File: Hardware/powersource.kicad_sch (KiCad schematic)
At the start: 39 parts, among them J10 USB_C_Receptacle_USB2.0_16P, J14 Conn_01x01_Socket, J15 Conn_01x01_Socket, J6 Conn_01x01_Socket, J9 Conn_01x01_Socket, Q2 DMP3015LSS-13, SW1 SW_Push_DPDT, U4 TPS61022, U8 CN3158

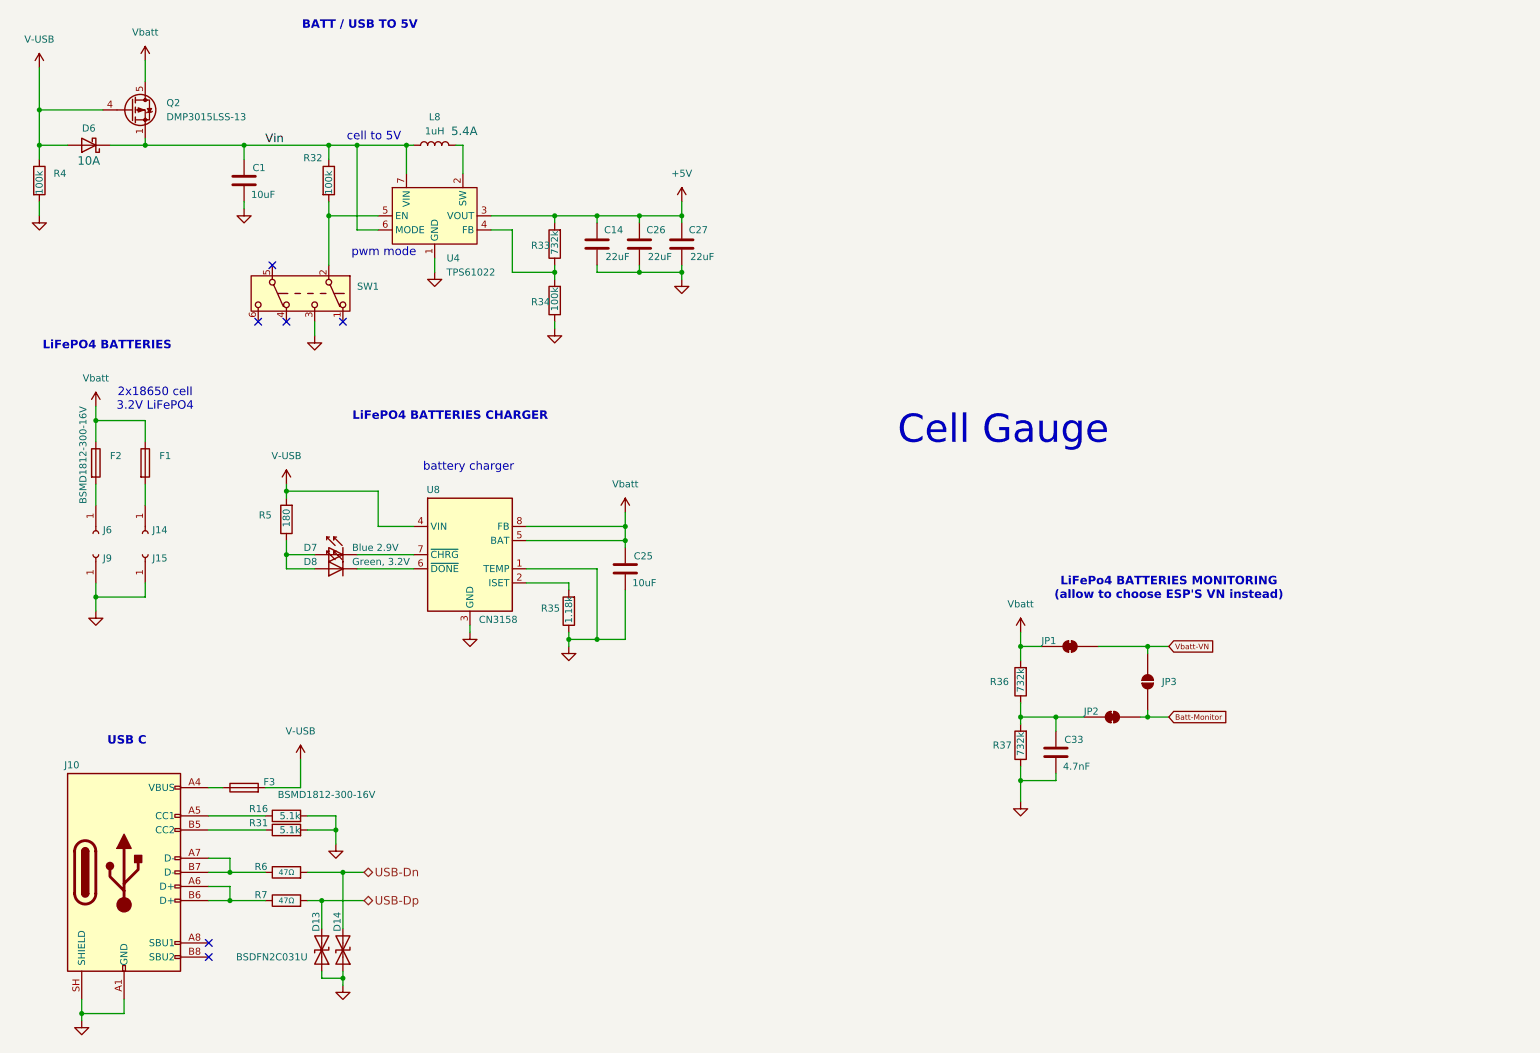
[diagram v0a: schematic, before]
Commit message: Schematic Done
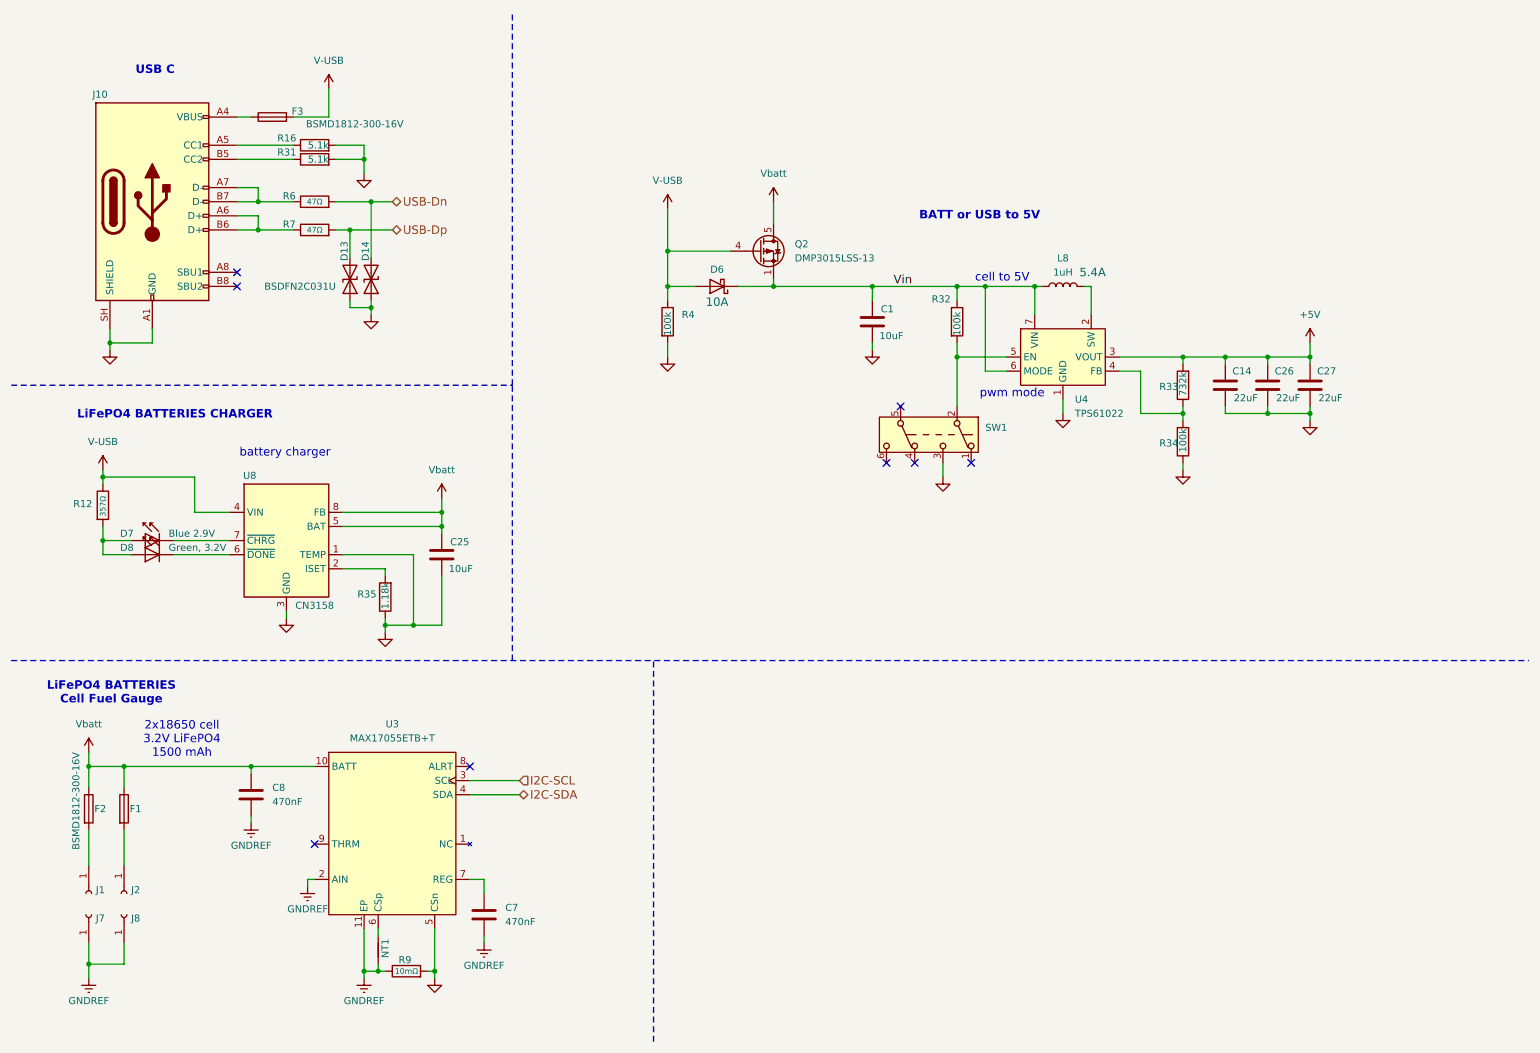
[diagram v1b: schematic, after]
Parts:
- removed C33: 4.7nF, Capacitor_SMD:C_0402_1005Metric, symbol Device:C
- removed JP1, JP2: SolderJumper_2_Bridged, Jumper:SolderJumper-2_P1.3mm_Bridged_Pad1.0x1.5mm, symbol Jumper:SolderJumper_2_Bridged
- removed JP3: SolderJumper_2_Open, Jumper:SolderJumper-2_P1.3mm_Open_TrianglePad1.0x1.5mm, symbol Jumper:SolderJumper_2_Open
- removed R36, R37: 732k, Resistor_SMD:R_0402_1005Metric, symbol Device:R
- removed R5: 180, Resistor_SMD:R_0402_1005Metric, symbol Device:R
- added C7, C8: 470nF, Capacitor_SMD:C_0402_1005Metric, symbol YV-library:CAPX470NM16V0-00
- added NT1: NetTie_2, NetTie:NetTie-2_SMD_Pad0.5mm, symbol Device:NetTie_2
- added R12: 357Ω, Resistor_SMD:R_0603_1608Metric, symbol YV-library:RES357RM-00
- added R9: 10mΩ, Resistor_SMD:R_1206_3216Metric, symbol YV-library:RESR010M-00
- added U3: MAX17055ETB+T, YV:TDFN-10-EP-2x2p5-0p4mm, symbol YV-library:MAX17055
- renumbered J6 to J1, J14 to J2, J9 to J7, J15 to J8
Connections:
- net GND: now also R9.2, U3.5 (CSn); no longer J7.1 (Pin_1), J8.1 (Pin_1)
- net V-USB: now also R12.1
- net Vbatt: now also C8.2, U3.10 (BATT)
- net at D7.2 (A), D8.2 (A): now also R12.2
- new net: NT1.2, U3.6 (CSp)
- new net: C7.2, U3.7 (REG)
- new net GNDREF: C7.1, C8.1, J7.1 (Pin_1), J8.1 (Pin_1), NT1.1, R9.1, U3.11 (EP), U3.2 (AIN)
- new net I2C-SCL: U3.3 (SCL)
- new net I2C-SDA: U3.4 (SDA)
- no-connect marks 6 -> 8
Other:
- note added: "2x18650 cell 3.2V LiFePO4 1500 mAh"
- note added: "BATT or USB to 5V"
- note added: "LiFePO4 BATTERIES Cell Fuel Gauge"
- note removed: "2x18650 cell 3.2V LiFePO4"
- note removed: "BATT / USB TO 5V"
- note removed: "Cell Gauge"
- note removed: "LiFePO4 BATTERIES"
- note removed: "LiFePo4 BATTERIES MONITORING (allow to choose ESP'S VN instead)"
- company: (none) -> Motion Composites
- title: (none) -> Strain Gauge Data Logger
- moved on the sheet: C1, C14, C25, C26, C27, D13, D14, D6, D7, D8, F1, F2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
